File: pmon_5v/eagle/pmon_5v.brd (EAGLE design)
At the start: 60 x 60 mm, 30 parts, among them J1 USB, J2 USB, J4 USB_A, J5 PINHD-2X3, Q1 16Mhz, U1 LTC2943, U2 FT232RL, U4 ATMEGA328TQFP32

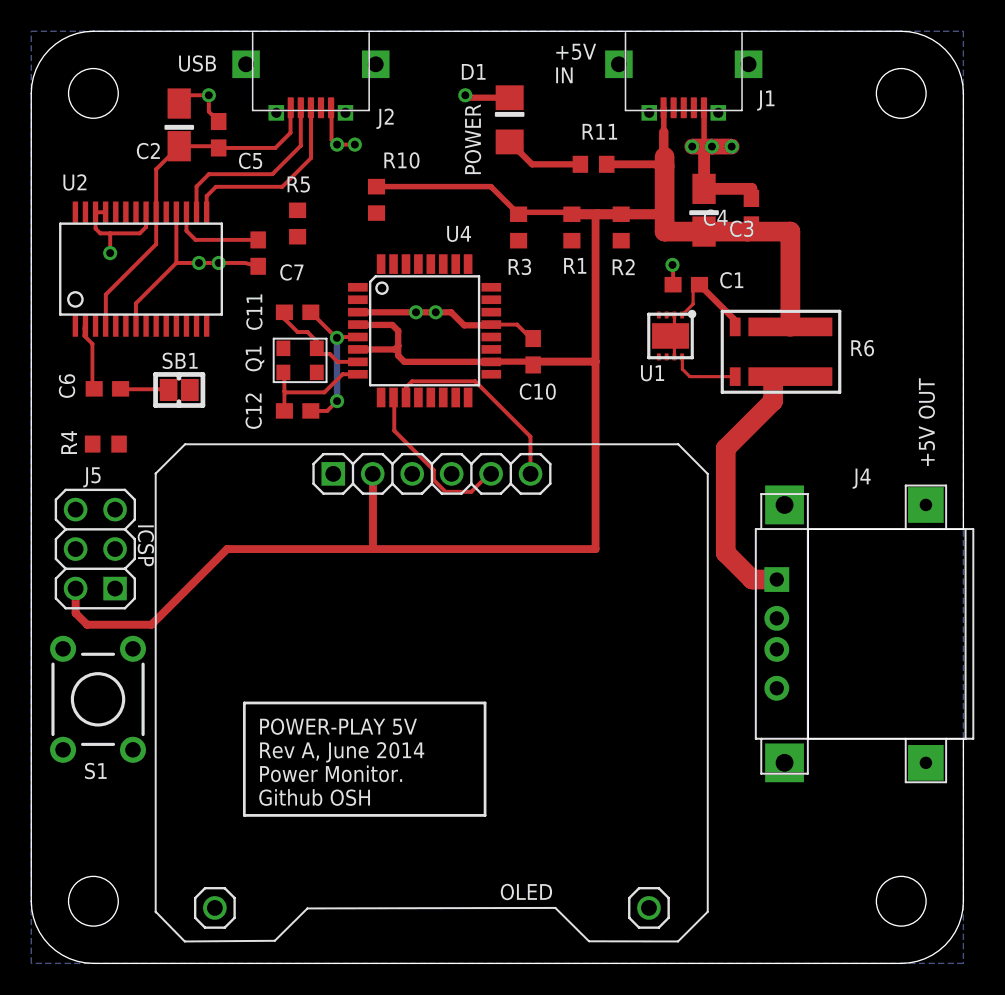
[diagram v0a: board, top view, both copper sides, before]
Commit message: Performed the final auto routing.
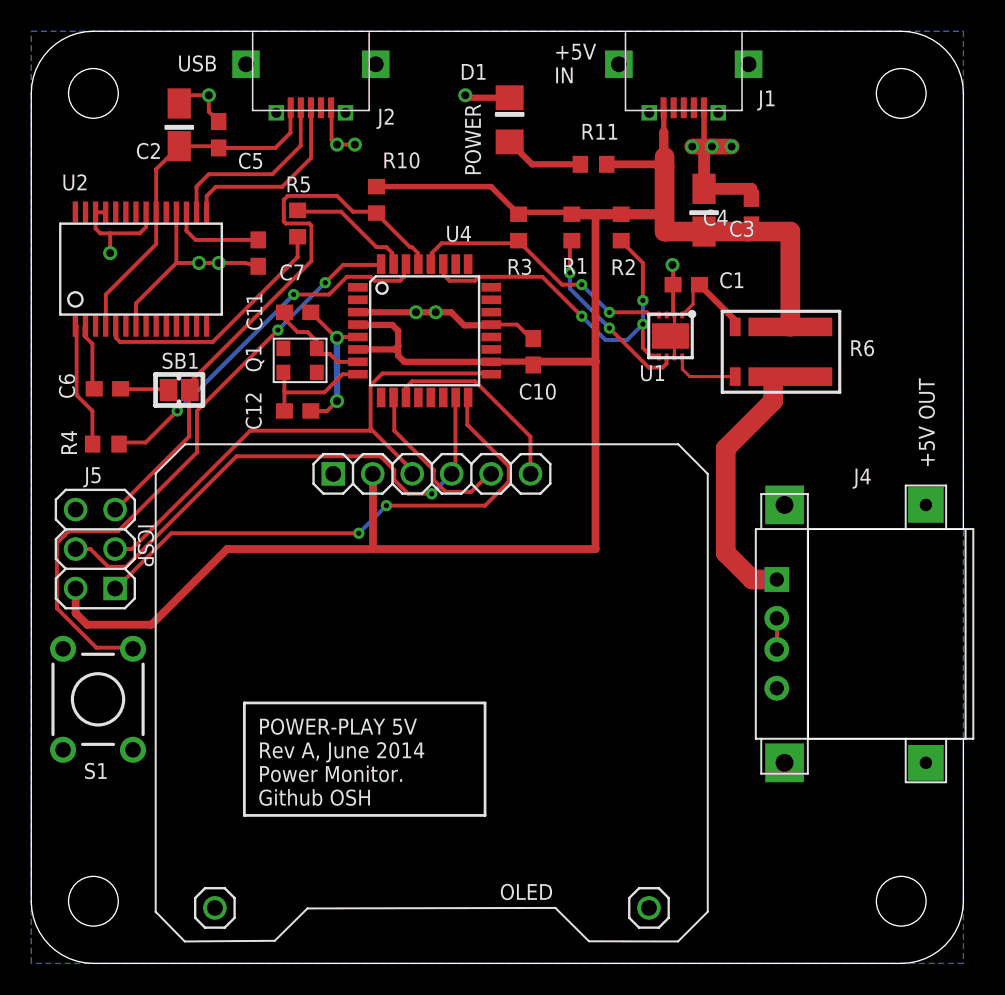
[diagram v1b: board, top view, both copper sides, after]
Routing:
- net START: track 0.00 -> 40.0 mm, vias 0 -> 2
- net RESET: track 0.00 -> 37.9 mm
- net MISO: track 0.12 -> 34.8 mm, vias 0 -> 2
- net SCK: track 0.30 -> 34.9 mm
- net MOSI: track 0.11 -> 34.7 mm, vias 0 -> 1
- net I2C-DATA: track 0.00 -> 24.7 mm, vias 0 -> 3
- net SER_RX: track 0.00 -> 23.9 mm, vias 0 -> 2
- net I2C-CLK: track 0.13 -> 17.9 mm, vias 0 -> 2
- net N$8: track 0.00 -> 16.1 mm
- net N$1: track 0.05 -> 12.0 mm, vias 0 -> 2
- net N$6: track 0.00 -> 8.10 mm
- net SER_TX: track 0.00 -> 8.03 mm
- net GND: track 72.2 -> 74.4 mm
- net N$4: track 0.00 -> 2.00 mm
